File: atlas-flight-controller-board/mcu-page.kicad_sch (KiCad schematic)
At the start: 1 part, among them U2 DEV-16771

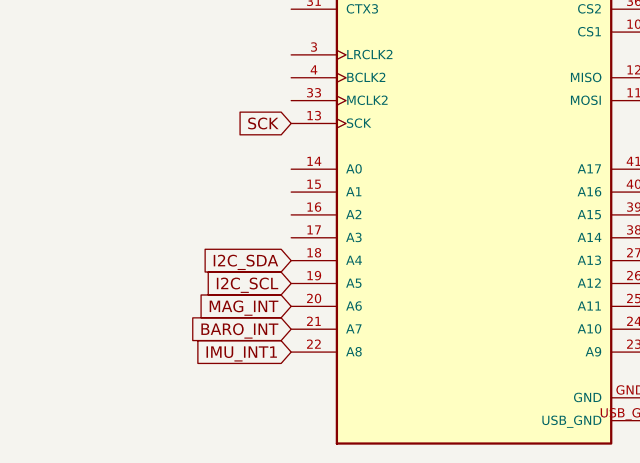
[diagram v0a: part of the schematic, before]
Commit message: Wip commit
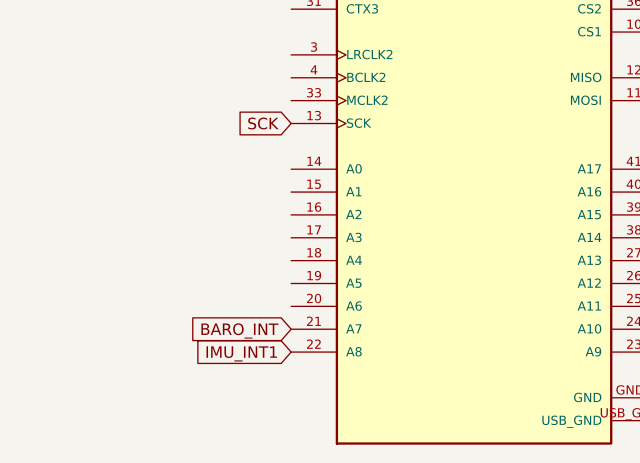
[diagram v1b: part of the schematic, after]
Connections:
- net I2C_SCL: no longer names the net of U2.19 (A5)
- net I2C_SDA: no longer names the net of U2.18 (A4)
- net MAG_INT: no longer names the net of U2.20 (A6)
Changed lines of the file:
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@@
-		)
-	)
-	(global_label "MAG_INT"
-		(shape input)
-		(at 124.46 124.46 180)
-		(fields_autoplaced yes)
-		(effects
-			(font
-				(size 1.27 1.27)
-			)
-			(justify right)
-		)
-		(property "Intersheetrefs" "${INTERSHEET_REFS}"
-			(at 113.7943 124.46 0)
-			(effects
-				(font
-					(size 1.27 1.27)
-				)
-				(justify right)
-				(hide yes)
-			)
 		)
 	)
@@
 		)
 	)
-	(global_label "I2C_SDA"
-		(shape input)
-		(at 124.46 119.38 180)
-		(fields_autoplaced yes)
-		(effects
-			(font
-				(size 1.27 1.27)
-			)
-			(justify right)
-		)
-		(property "Intersheetrefs" "${INTERSHEET_REFS}"
-			(at 113.8548 119.38 0)
-			(effects
-				(font
-					(size 1.27 1.27)
-				)
-				(justify right)
-				(hide yes)
-			)
-		)
-	)
 	(global_label "BARO_INT"
 		(shape input)
@@
 			(effects
 				(font
-					(size 1.27 1.27)
-				)
-				(justify right)
-				(hide yes)
-			)
-		)
-	)
-	(global_label "I2C_SCL"
-		(shape input)
-		(at 124.46 121.92 180)
-		(fields_autoplaced yes)
-		(effects
-			(font
-				(size 1.27 1.27)
-			)
-			(justify right)
-		)
-		(property "Intersheetrefs" "${INTERSHEET_REFS}"
-			(at 113.9153 121.92 0)
-			(effects
-				(font
